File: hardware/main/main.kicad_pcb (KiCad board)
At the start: 4 copper layers, 21 x 55.9 mm, 70 parts, among them J1 Conn_ARM_SWD_TagConnect_TC203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, J101 CHAIN OUT, J103 NTC (optional), J2 USB4105-GF-A, J200 PROTECTED CELL 90mAh, M1 VLV041235L, Q1 2N7002, SW1 ESP RESET, SW2 ESP BOOT, SW3 WAKE / SHIP, U1 ESP32-C6-MINI-1, U11 BQ25186DLH, U12 TPS63802DLA, U14 TPD2EUSB30, U15 TPD2EUSB30, U18 M2003FC1AE, U26 TPS22918DBV, U3 DRV2625

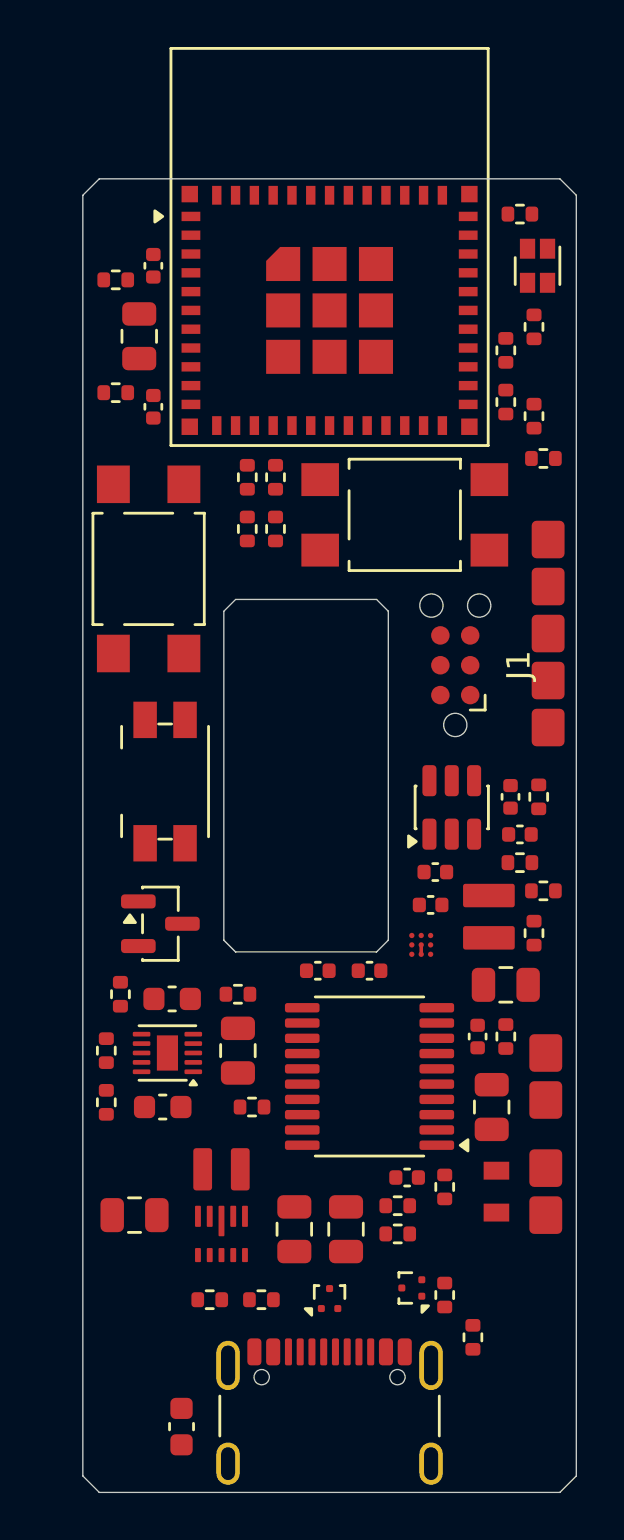
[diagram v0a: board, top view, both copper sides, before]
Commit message: PCB housing
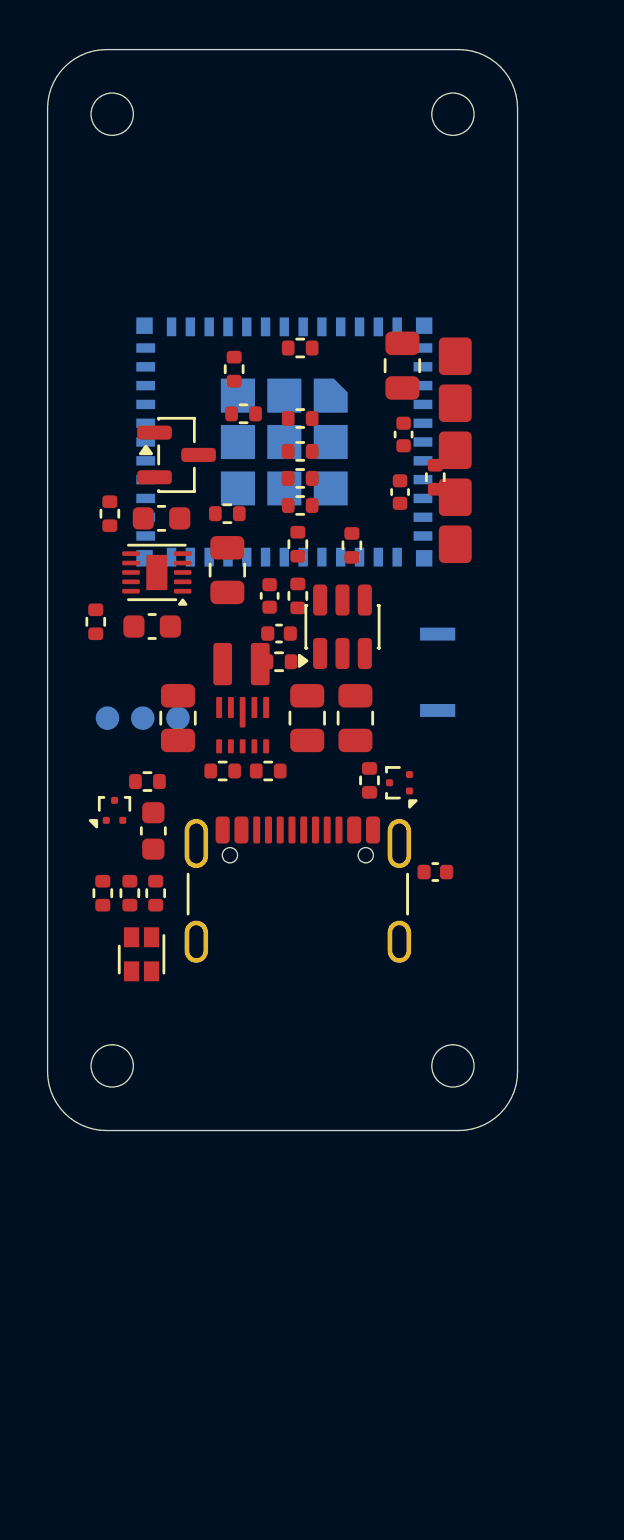
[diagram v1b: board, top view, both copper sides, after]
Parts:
- removed C100, C5, C6: 100n, Capacitor_SMD:C_0402_1005Metric
- removed C101: 10u, Capacitor_SMD:C_0805_2012Metric
- removed C102: 10n, Capacitor_SMD:C_0402_1005Metric
- removed C103: 22u 10V X5R, Capacitor_SMD:C_0805_2012Metric
- removed C7: 1u, Capacitor_SMD:C_0402_1005Metric
- removed F100: 250mA FAST, HapticBracelet:Fuse_Littelfuse_467_0603
- removed J1: Conn_ARM_SWD_TagConnect_TC2030-NL, Connector:Tag-Connect_TC2030-IDC-NL_2x03_P1.27mm_Vertical
- removed J103: NTC (optional), HapticBracelet:WirePads_2_P2mm
- removed J200: PROTECTED CELL 90mAh, HapticBracelet:WirePads_2_P2mm
- removed M1: VLV041235L, HapticBracelet:Vybronics_VLV041235L_FPC_Contact_Draft
- removed R100: 0, Resistor_SMD:R_0402_1005Metric
- removed R101: 33, Resistor_SMD:R_0402_1005Metric
- removed R102, R103: 100k, Resistor_SMD:R_0402_1005Metric
- removed R105: 10k 1%, Resistor_SMD:R_0402_1005Metric
- removed R8, R9: 4.7k, Resistor_SMD:R_0402_1005Metric
- removed SW1: ESP RESET, Button_Switch_SMD:SW_SPST_TL3305A
- removed SW2: ESP BOOT, Button_Switch_SMD:SW_SPST_TL3305A
- removed U18: M2003FC1AE, Package_SO:TSSOP-20_4.4x6.5mm_P0.65mm
- removed U3: DRV2625, HapticBracelet:DRV2625_YFF_9_0.4mm
- added H1: M1.6 CLEARANCE, HapticBracelet:Screw_Clearance_M1p6_1p8mm_Stack, F.Cu at (36.2, 37.4)
- added H2: M1.6 CLEARANCE, HapticBracelet:Screw_Clearance_M1p6_1p8mm_Stack, F.Cu at (50.8, 37.4)
- added H3: M1.6 CLEARANCE, HapticBracelet:Screw_Clearance_M1p6_1p8mm_Stack, F.Cu at (36.2, 77.8)
- added H4: M1.6 CLEARANCE, HapticBracelet:Screw_Clearance_M1p6_1p8mm_Stack, F.Cu at (50.8, 77.8)
- added J3: ESP RECOVERY, HapticBracelet:ESP_Recovery_3Pads_P1.5mm, B.Cu at (37.5, 63.0)
- J101: value CHAIN OUT -> STACK TO POD 0
- SW3: footprint Button_Switch_SMD:Panasonic_EVQPUJ_EVQPUA -> HapticBracelet:SW_SPST_Panasonic_EVPAW_3x2mm_H0.6mm; moved to B.Cu
- U1: moved to B.Cu
- moved D1 33.8 mm to (37.5, 73.1)
- moved R47 33.3 mm to (37.0, 70.5), turned to -90 degrees
- moved R49 29.0 mm to (38.1, 70.5), turned to -90 degrees
- moved C32 25.4 mm to (38.0, 67.8)
- moved R60 25.2 mm to (37.8, 65.8), turned to 180 degrees
- moved R61 24.1 mm to (47.2, 65.7)
- moved U14 22.7 mm to (36.4, 67.0)
- moved R41 22.5 mm to (41.0, 65.3)
- moved R40 22.5 mm to (42.9, 65.3)
- moved J2 22.3 mm to (44.1, 71.5)
- moved C38 21.8 mm to (44.5, 63.0)
- moved C39 21.8 mm to (46.6, 63.0)
- moved U12 21.7 mm to (41.8, 63.4)
- moved L1 21.5 mm to (41.8, 60.8)
- moved U15 21.5 mm to (48.5, 65.8)
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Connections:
- J101 pad 3: RING_D1 -> RING_D0
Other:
- board size 21 x 55.9 mm -> 20 x 46 mm
- board text added: "20 x 46 mm POD FACE / R2.5 Cmts.User: TPU contact inner edge, 1.2 mm inset Dwgs.User dashed: placement limit, 1.5 mm inset Corner circles: D4.6 TPU standoff relief Height / screw length TBD; drawings are not copper keepouts"
